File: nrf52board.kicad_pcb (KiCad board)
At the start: 2 copper layers, 27.9 x 59.7 mm, 47 parts, among them J1 Conn_01x04, J2 USB_B_Micro, J3 Battery, Q1 Q_PMOS_DSG, SW1 SW_Push, SW2 SW_Push, U1 nrf52board, U2 E73-2G4M04S, U3 MCP73831-2-OT, U4 LP2985-3.3, U5 RFM95W-868S2, U6 CP2102-GM

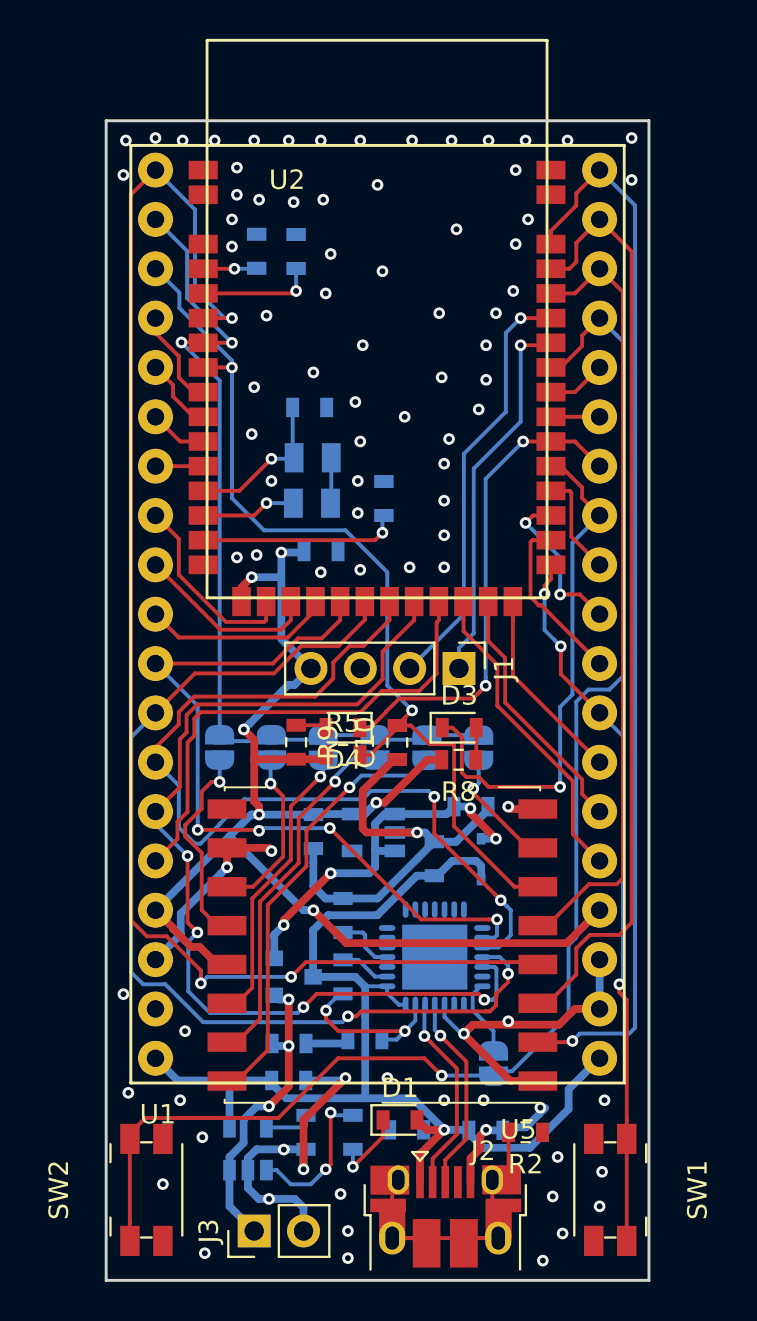
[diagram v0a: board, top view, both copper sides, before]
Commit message: pcb: done
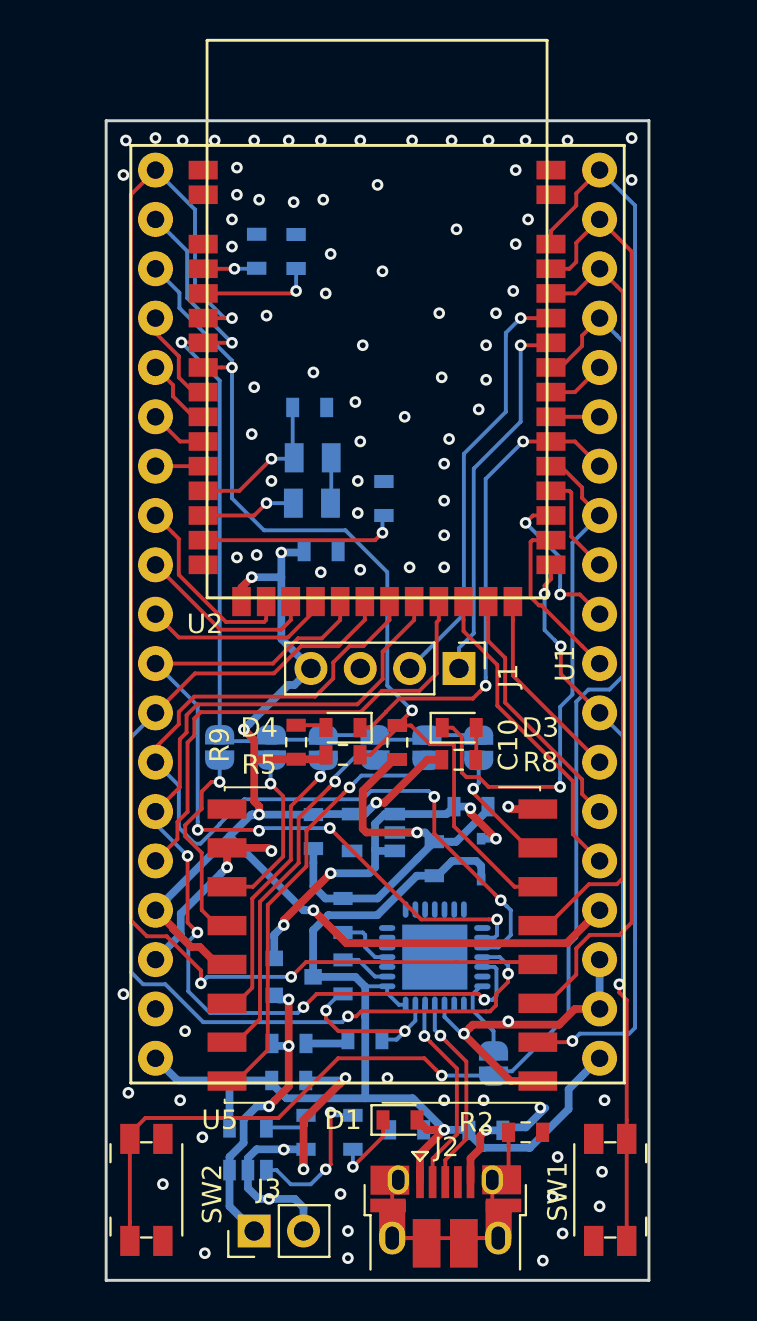
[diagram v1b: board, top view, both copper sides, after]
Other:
- board text added: "github.com/ dimka-rs/ nrf52board rev.1"
